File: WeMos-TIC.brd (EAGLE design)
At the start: 33.2 x 25.7 mm, 22 parts, among them Q2 BSS138

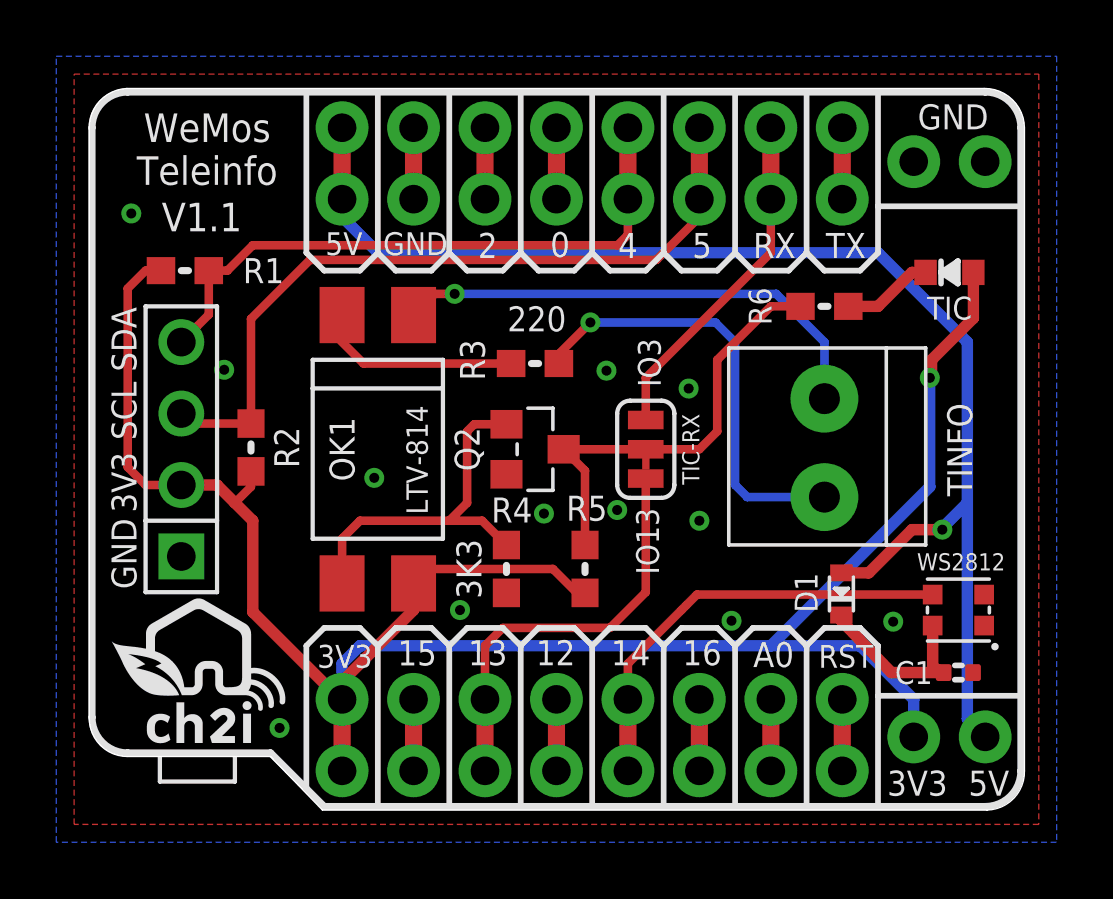
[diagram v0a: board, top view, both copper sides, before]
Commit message: Bump to v1.2
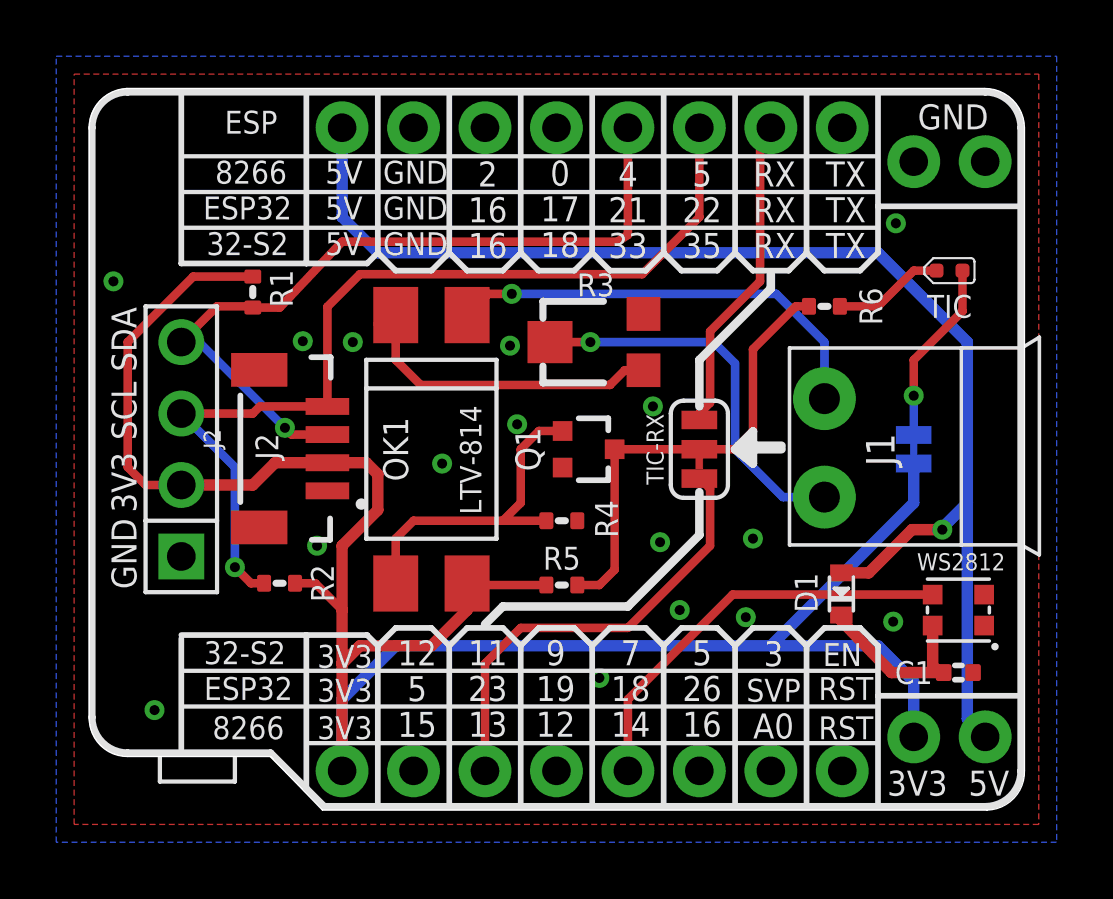
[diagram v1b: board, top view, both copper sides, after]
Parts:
- removed JP7, JP8: (no value), SparkFun-Connectors:1X08_NO_SILK
- removed Q2: BSS138, Seeed-Discrete:SOT23
- removed TINFO: 1X2-3.5MM, adafruit:1X2-3.5MM
- removed U$2: (no value), _c2h:LOGO_C2I_015
- added J1: KF2EDGR-3.81-2P, _c2h:1X2-3.5MM
- added J2: Qwiic Connector, _c2h:JST04_1MM_VERT
- added JLED: (no value), SparkFun-Passives:PAD-JUMPER-2-NC_BY_TRACE_YES_SILK
- added Q1: BSS138, _c2h:SOT-323-3
- R1, R2, R4, R5, R6: device _c2h:0603-RES -> _c2h:0402-RES
- R3: value 220 -> 2K; device _c2h:0603-RES -> adafruit:TC33X
- TIC: value (none) -> BLUE; device _c2h:0603-LED -> OPL_Optoelectronics:LED-0402
- moved R2 4.93 mm to (6.67, 7.94), turned to 0 degrees
- moved R4 2.61 mm to (16.7, 10.2), turned to 180 degrees
- moved R1 2.53 mm to (5.71, 18.3), turned to 90 degrees
- moved R3 2.17 mm to (17.8, 16.5), turned to 90 degrees
- moved RX 1.91 mm to (21.6, 12.7)
- moved OK1 1.90 mm to (12.1, 12.7)
- moved R5 1.00 mm to (16.7, 7.87), turned to 180 degrees
- moved TIC 0.06 mm to (30.5, 19.1), turned to 180 degrees
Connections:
- new net LTIC: JLED.2, TIC.+
- net 3V3: now also J2.2, JLED.1; no longer JP7.8, TIC.PLUS
- net 5V: no longer JP8.8
- net A0: no longer JP7.2
- net GND: now also J2.1, Q1.2; no longer JP8.7, Q2.2
- net GPIO0: no longer JP8.5
- net GPIO1: no longer JP8.1
- net GPIO12: no longer JP7.5
- net GPIO13: no longer JP7.6
- net GPIO14: no longer JP7.4
- net GPIO16: no longer JP7.3
- net GPIO2: no longer JP8.6
- net GPIO3: no longer JP8.2
- net N$1: now also TIC.-; no longer TIC.MINUS
- net N$2: now also Q1.1; no longer Q2.1
- net N$4: now also J1.1; no longer TINFO.1
- net N$5: now also J1.2; no longer TINFO.2
- net RST: no longer JP7.1
- net SCL: now also J2.4; no longer JP8.3
- net SDA: now also J2.3; no longer JP8.4
- net SS: no longer JP7.7
- net TIC-RX: now also Q1.3; no longer Q2.3
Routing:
- net SCL: track 27.1 -> 34.1 mm, vias 0 -> 1
- net LTIC: track 0.00 -> 6.56 mm, vias 0 -> 1
- net SDA: track 23.0 -> 27.9 mm, vias 0 -> 1
- net N$3: track 7.99 -> 11.8 mm
- net SS: track 2.54 -> 0.00 mm
- net RST: track 2.54 -> 0.00 mm
- net GPIO16: track 2.54 -> 0.00 mm
- net GPIO12: track 2.54 -> 0.00 mm
- net A0: track 2.54 -> 0.00 mm
- net GPIO2: track 2.54 -> 0.00 mm
- net GPIO1: track 2.54 -> 0.00 mm
- net GPIO0: track 2.54 -> 0.00 mm
- net GND: track 2.54 -> 0.00 mm, vias 12 -> 16
- net N$5: track 15.8 -> 13.8 mm
- net N$4: track 17.6 -> 15.7 mm
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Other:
- board text added: "1"
- board text added: "10"
- board text added: "11"
- board text added: "17"
- board text added: "18"
- board text added: "19"
- board text added: "21"
- board text added: "22"
- board text added: "23"
- board text added: "26"
- board text added: "3"
- board text added: "32-C3"
- board text added: "32-S2"
- board text added: "32-S3"
- board text added: "33"
- board text added: "35"
- board text added: "36"
- board text added: "6"
- board text added: "7"
- board text added: "8"
- board text added: "8266"
- board text added: "9"
- board text added: "Cut to disable Teleinfo LED"
- board text added: "EN"
- board text added: "ESP"
- board text added: "ESP32"
- board text added: "J2"
- board text added: "SVP"
- board text added: "V1.2"
- board text added: "hallard.me"
- board text removed: "IO13"
- board text removed: "IO3"
- board text removed: "V1.1"
